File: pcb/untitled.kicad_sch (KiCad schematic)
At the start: 48 parts, among them IC10 AD844_OPAMP_MEL, IC3 FOD814_OPTO_NOSHD, IC5 FOD814_OPTO_MEL, IC6 AD844_OPAMP_AL, IC7 FOD814_OPTO_AL, IC8 AD844_OPAMP_NOSHD, U2 REF192_NOSHD, U3 REF192_AL, U4 REF192_MEL

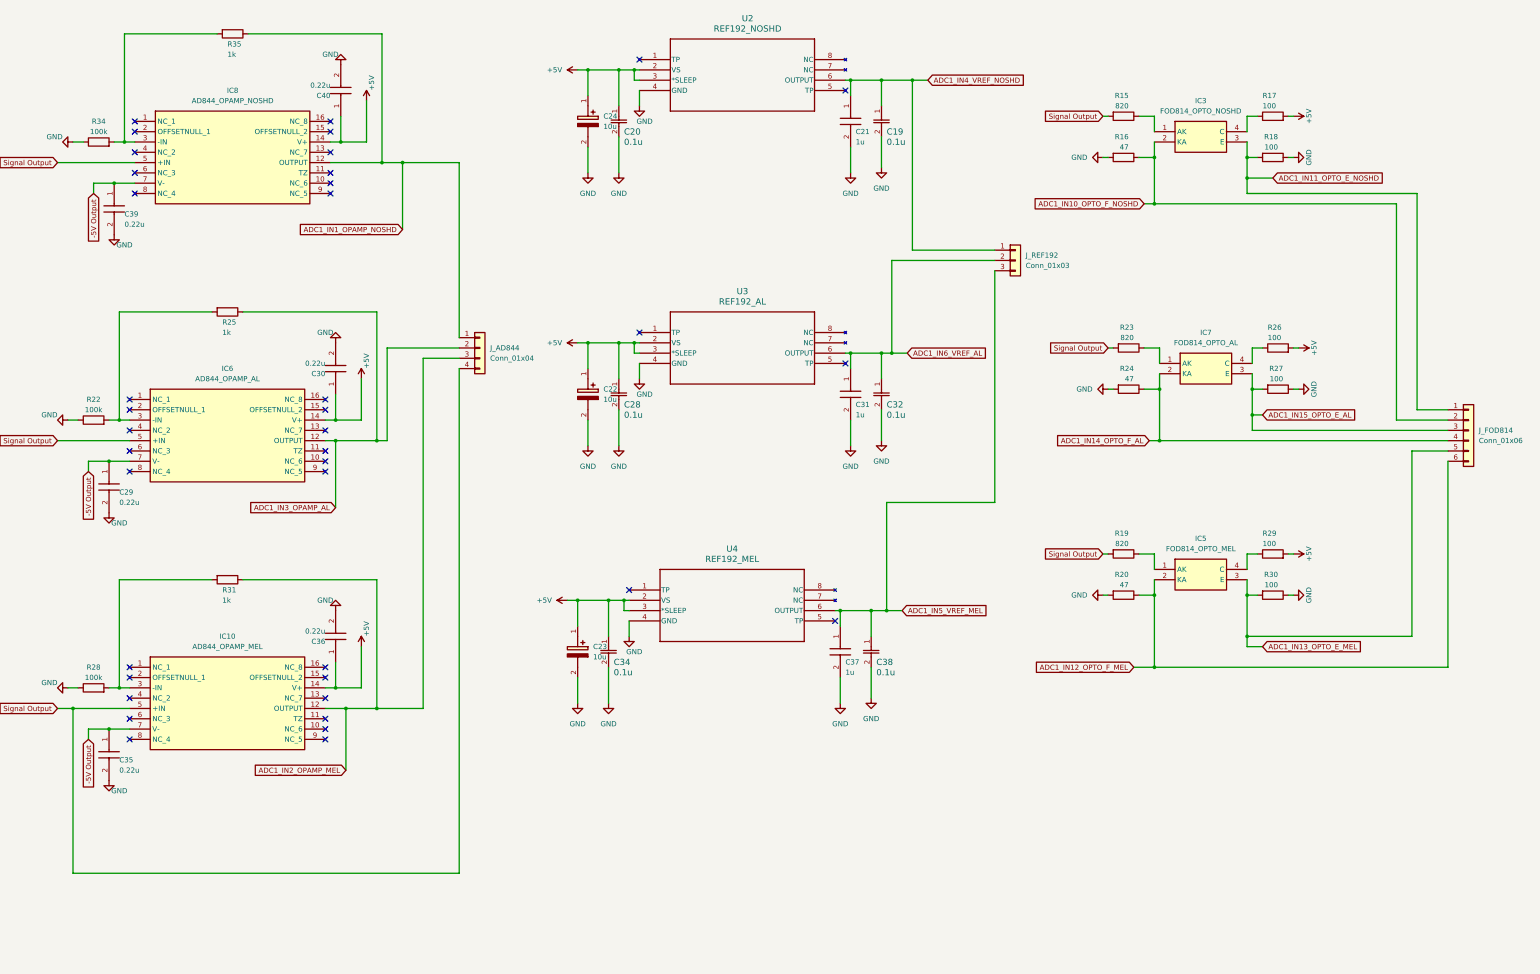
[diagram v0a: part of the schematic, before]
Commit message: Working Commit - Nov24
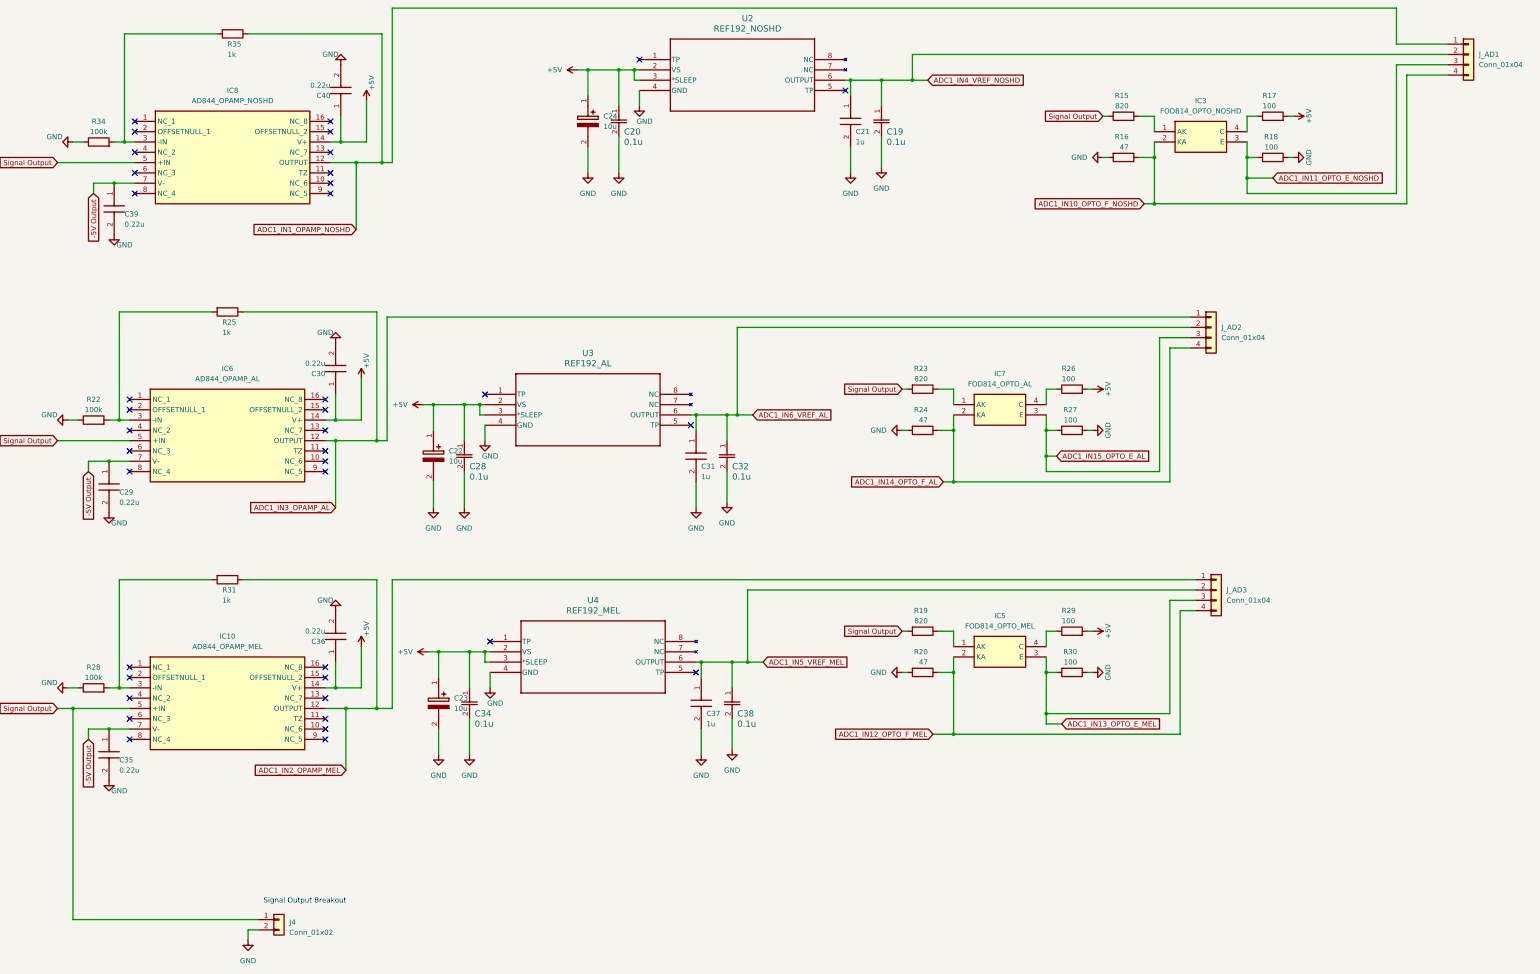
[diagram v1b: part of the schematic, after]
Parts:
- removed J_AD844: Conn_01x04, Connector_PinHeader_2.54mm:PinHeader_1x04_P2.54mm_Vertical, symbol Connector_Generic:Conn_01x04
- removed J_FOD814: Conn_01x06, Connector_PinHeader_2.54mm:PinHeader_1x06_P2.54mm_Vertical, symbol Connector_Generic:Conn_01x06
- removed J_REF192: Conn_01x03, Connector_PinHeader_2.54mm:PinHeader_1x03_P2.54mm_Vertical, symbol Connector_Generic:Conn_01x03
- added J4: Conn_01x02, Connector_PinHeader_2.54mm:PinHeader_1x02_P2.54mm_Vertical, symbol Connector_Generic:Conn_01x02
- added J_AD1, J_AD2, J_AD3: Conn_01x04, Connector_PinHeader_2.54mm:PinHeader_1x04_P2.54mm_Vertical, symbol Connector_Generic:Conn_01x04
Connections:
- net ADC1_IN10_OPTO_F_NOSHD: now also J_AD1.4 (Pin_4)
- net ADC1_IN11_OPTO_E_NOSHD: now also J_AD1.3 (Pin_3)
- net ADC1_IN12_OPTO_F_MEL: now also J_AD3.4 (Pin_4)
- net ADC1_IN13_OPTO_E_MEL: now also J_AD3.3 (Pin_3)
- net ADC1_IN14_OPTO_F_AL: now also J_AD2.4 (Pin_4)
- net ADC1_IN15_OPTO_E_AL: now also J_AD2.3 (Pin_3)
- net ADC1_IN1_OPAMP_NOSHD: now also J_AD1.1 (Pin_1)
- net ADC1_IN2_OPAMP_MEL: now also J_AD3.1 (Pin_1)
- net ADC1_IN3_OPAMP_AL: now also J_AD2.1 (Pin_1)
- net ADC1_IN4_VREF_NOSHD: now also J_AD1.2 (Pin_2)
- net ADC1_IN5_VREF_MEL: now also J_AD3.2 (Pin_2)
- net ADC1_IN6_VREF_AL: now also J_AD2.2 (Pin_2)
- net GND: now also J4.2 (Pin_2)
- net Signal Output: now also J4.1 (Pin_1)
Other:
- note added: "Signal Output Breakout"
- moved on the sheet: C22, C23, C28, C31, C32, C34, C37, C38, IC5, IC7, R19, R20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
